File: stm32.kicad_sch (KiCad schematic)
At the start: 21 parts, among them J5 PROG, J6 HC-05, SW2 B3S-1000, U9 STM32G431KBT6

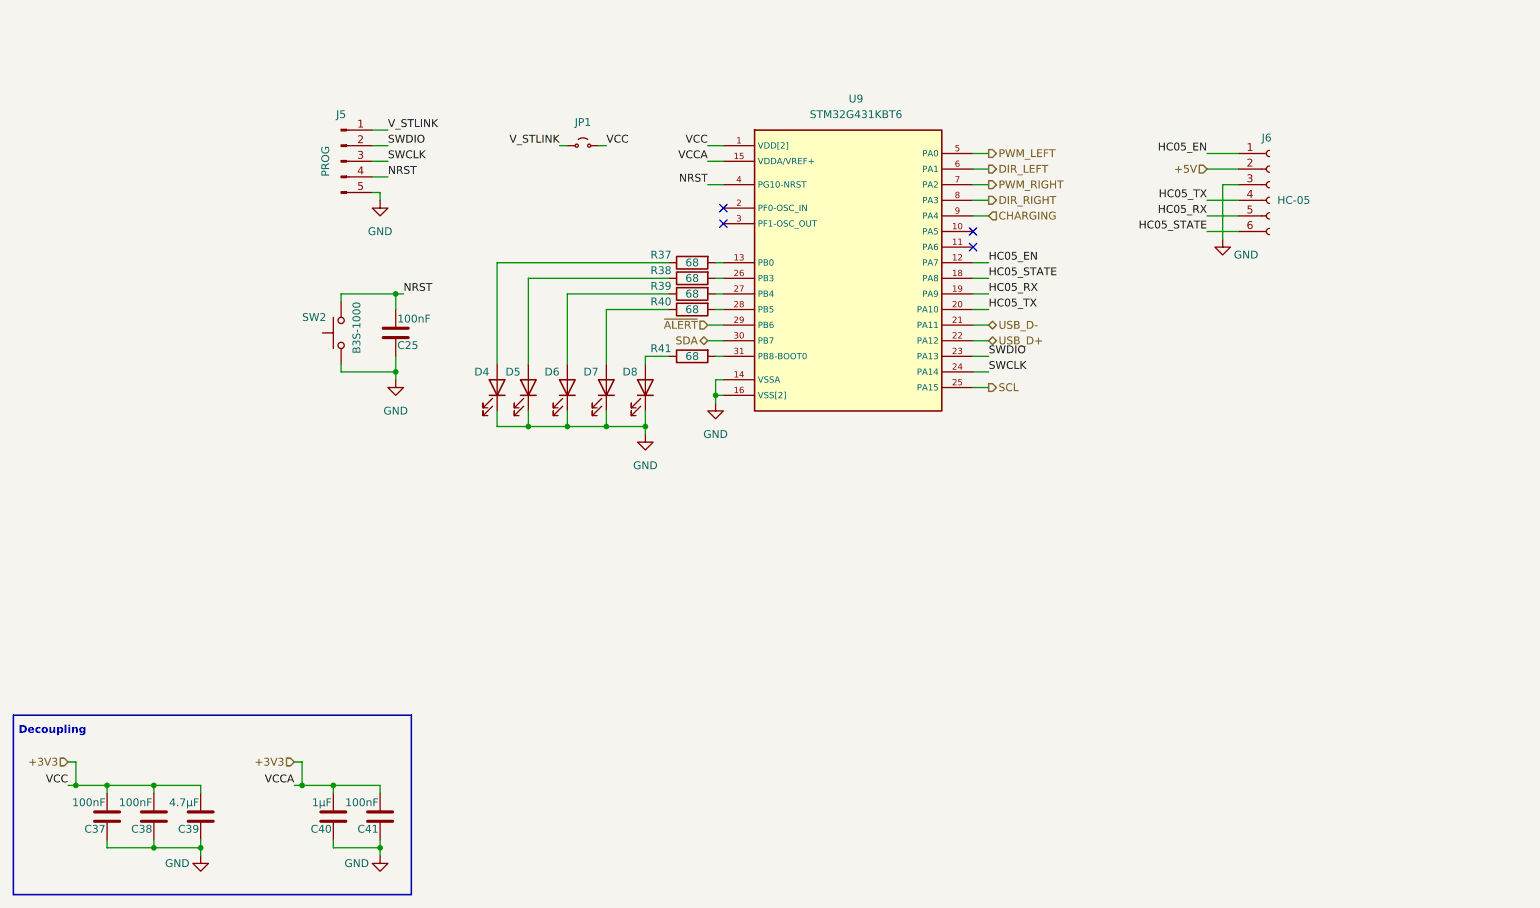
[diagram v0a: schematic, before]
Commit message: Minor Schematics update
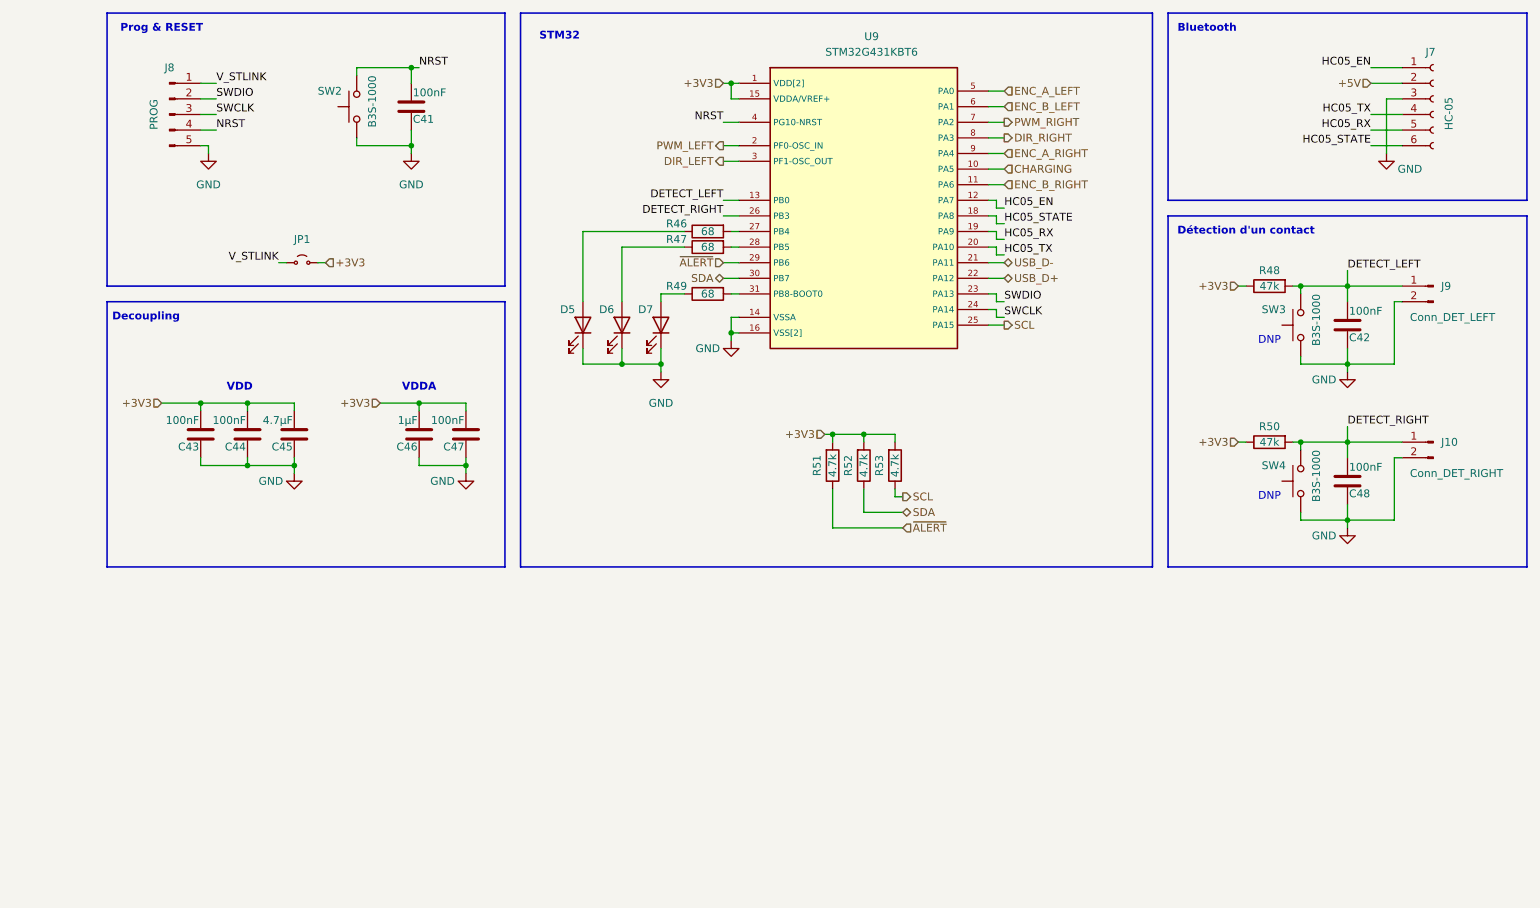
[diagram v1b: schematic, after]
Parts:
- removed D4, D5: LED, symbol Device:LED
- removed R37, R38: 68, Resistor_SMD:R_0805_2012Metric, symbol local:R
- added C42, C48: 100nF, Capacitor_SMD:C_0603_1608Metric, symbol local:C
- added J10: Conn_DET_RIGHT, Connector_PinHeader_2.54mm:PinHeader_1x02_P2.54mm_Vertical, symbol Connector:Conn_01x02_Pin
- added J9: Conn_DET_LEFT, Connector_PinHeader_2.54mm:PinHeader_1x02_P2.54mm_Vertical, symbol Connector:Conn_01x02_Pin
- added R48, R50: 47k, Resistor_SMD:R_0603_1608Metric, symbol local:R
- added R51, R52, R53: 4.7k, Resistor_SMD:R_0603_1608Metric, symbol local:R
- added SW3, SW4: B3S-1000, local:SW_SPST_B3S-1000, symbol Switch:SW_Push
- C41: renamed from C25; footprint Capacitor_SMD:C_0805_2012Metric -> Capacitor_SMD:C_0603_1608Metric; symbol local:C_0402 -> local:C
- C43: renamed from C37; footprint Capacitor_SMD:C_0805_2012Metric -> Capacitor_SMD:C_0603_1608Metric; symbol local:C_0402 -> local:C
- C44: renamed from C38; footprint Capacitor_SMD:C_0805_2012Metric -> Capacitor_SMD:C_0603_1608Metric; symbol local:C_0402 -> local:C
- C45: renamed from C39; symbol local:C_0402 -> local:C
- C46: renamed from C40; footprint Capacitor_SMD:C_0805_2012Metric -> Capacitor_SMD:C_0603_1608Metric; symbol local:C_0402 -> local:C
- C47: renamed from C41; footprint Capacitor_SMD:C_0805_2012Metric -> Capacitor_SMD:C_0603_1608Metric; symbol local:C_0402 -> local:C
- D5: renamed from D6; footprint (none) -> LED_SMD:LED_0603_1608Metric
- D6: renamed from D7; footprint (none) -> LED_SMD:LED_0603_1608Metric
- D7: renamed from D8; footprint (none) -> LED_SMD:LED_0603_1608Metric
- J7: renamed from J6; footprint (none) -> Connector_PinSocket_2.54mm:PinSocket_1x06_P2.54mm_Vertical
- J8: renamed from J5; footprint (none) -> Connector_PinHeader_2.54mm:PinHeader_1x05_P2.54mm_Vertical
- JP1: footprint (none) -> Connector_PinHeader_2.54mm:PinHeader_1x02_P2.54mm_Vertical
- R46: renamed from R39; footprint Resistor_SMD:R_0805_2012Metric -> Resistor_SMD:R_0603_1608Metric
- R47: renamed from R40; footprint Resistor_SMD:R_0805_2012Metric -> Resistor_SMD:R_0603_1608Metric
- R49: renamed from R41; footprint Resistor_SMD:R_0805_2012Metric -> Resistor_SMD:R_0603_1608Metric
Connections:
- net CHARGING: now also U9.10 (PA5); no longer U9.9 (PA4)
- net DIR_LEFT: now also U9.3 (PF1-OSC_OUT); no longer U9.6 (PA1)
- net GND: now also C42.1, C48.1, J10.2 (Pin_2), J9.2 (Pin_2), SW3.1, SW4.1
- net PWM_LEFT: now also U9.2 (PF0-OSC_IN); no longer U9.5 (PA0)
- net SCL: now also R53.1
- net SDA: now also R52.1
- net VDD: now also R48.1, R50.1, R51.2, R52.2, R53.2
- net ~{ALERT}: now also R51.1
- net DETECT_RIGHT: now reaches U9.26 (PB3)
- net DETECT_RIGHT: now also C48.2, J10.1 (Pin_1), R50.2, SW4.2
- net DETECT_LEFT: now reaches U9.13 (PB0)
- net DETECT_LEFT: now also C42.2, J9.1 (Pin_1), R48.2, SW3.2
- net ENC_B_RIGHT: now reaches U9.11 (PA6)
- new net ENC_A_LEFT: U9.5 (PA0)
- new net ENC_A_RIGHT: U9.9 (PA4)
- new net ENC_B_LEFT: U9.6 (PA1)
- no-connect marks 4 -> 0
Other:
- note added: "Bluetooth"
- note added: "DNP"
- note added: "Détection d'un contact"
- note added: "Prog & RESET"
- note added: "STM32"
- note added: "VDD"
- note added: "VDDA"
- moved on the sheet: C41, C43, C44, C45, C46, C47, D5, D6, D7, J7, J8, JP1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
